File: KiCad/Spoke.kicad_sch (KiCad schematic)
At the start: 134 parts, among them J1 B2B-PH-K-S, J10 BL-A, J11 BL-C, J12 Amphenol 132289, J2 BAT+, J3 BAT-, J4 GCT USB4105/USB4110, J5 USB+, J6 USB-, J7 PLS-1x3, J8 PLS-1x6, J9 PLS-1x3, Q1 AO3407A, Q2 AO3407A, Q3 AO3400, Q4 AO3400, Q5 AO3400, SW1 PWR, SW2 OK/UP, SW3 ESC/DN, SW4 BOOT, U1 SP0503BAHTG, U2 TP4056, U3 CP2102N-A02-GQFN28, U4 LM3671MF-3.3, U5 74HC4052PW, U6 STM32F103C8T6, U7 LSM303DLHC, X1 8MHz

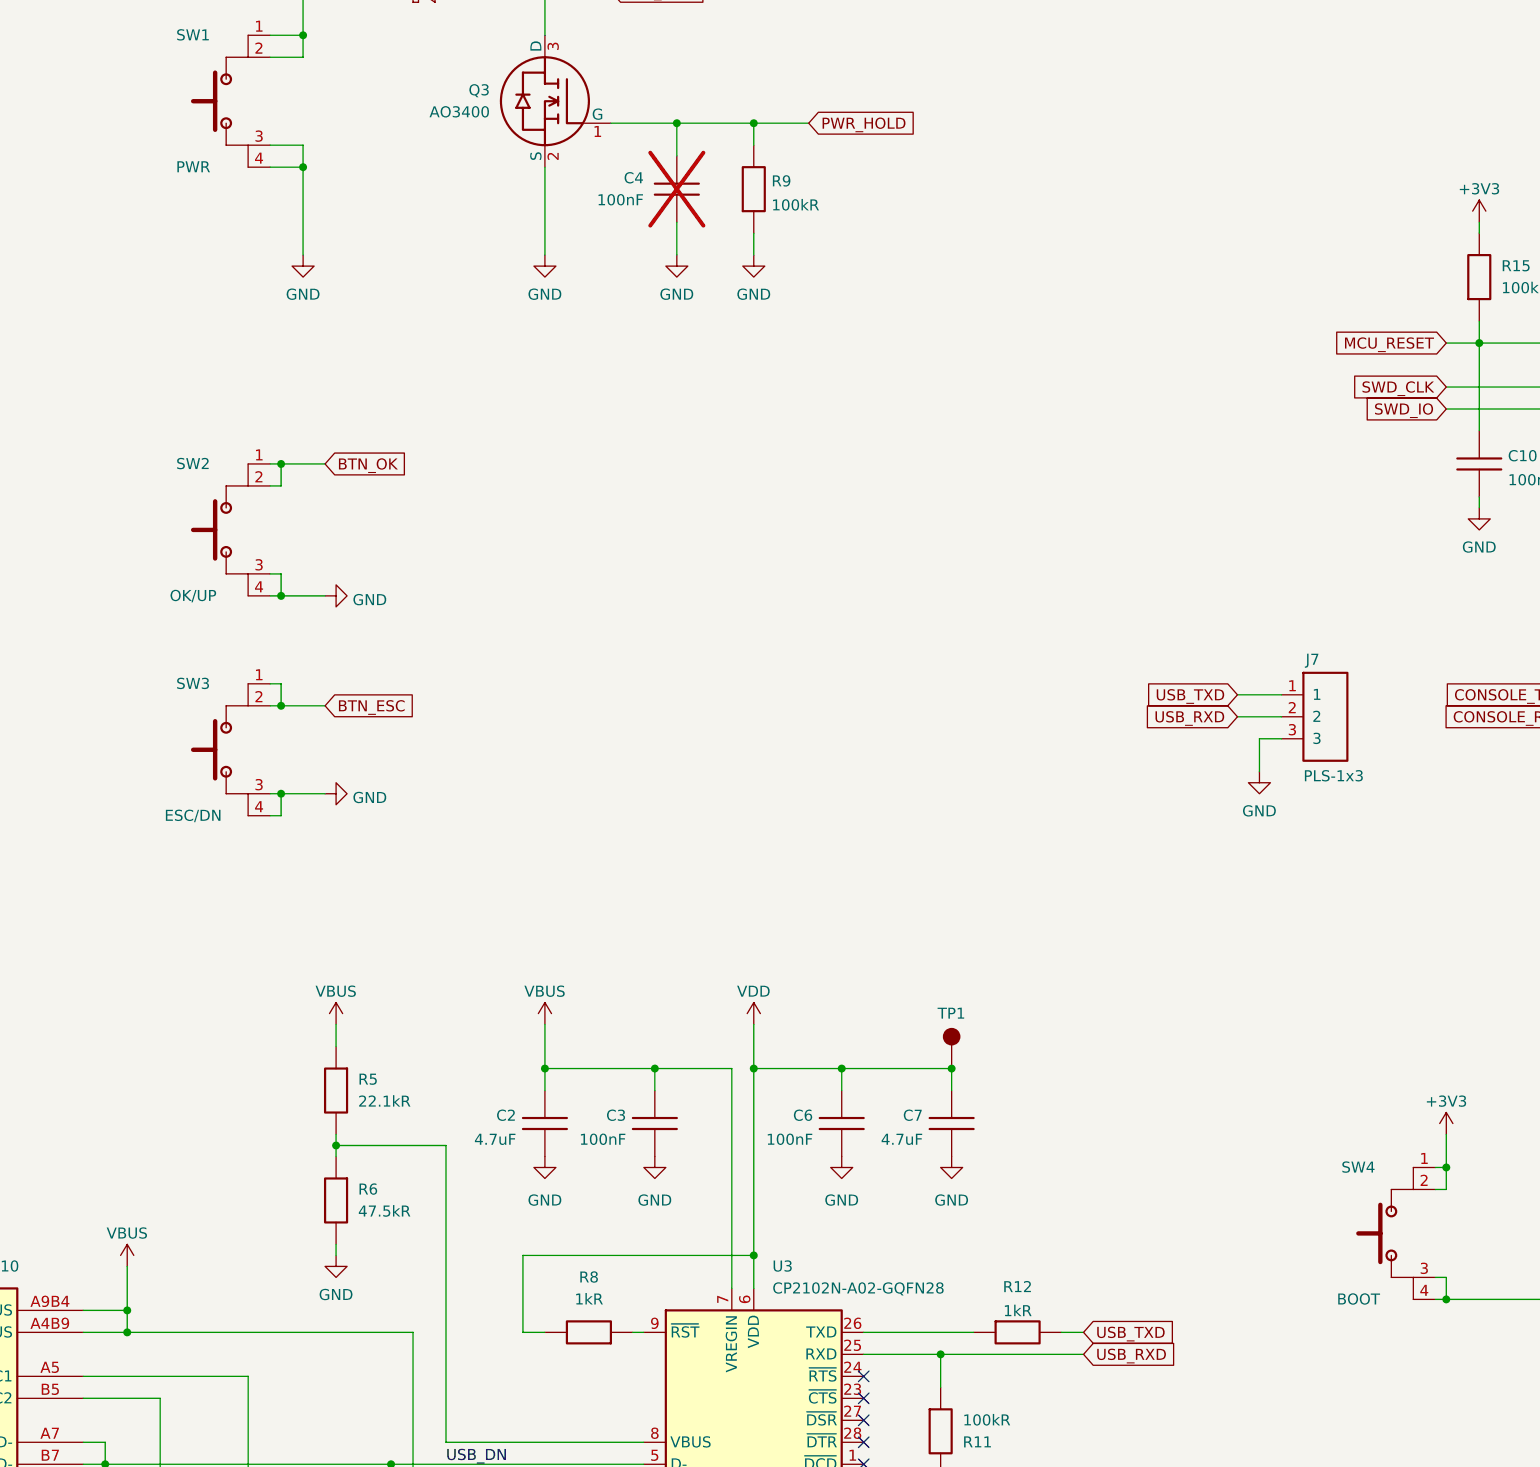
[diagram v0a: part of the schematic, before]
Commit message: Export SCH and BOM
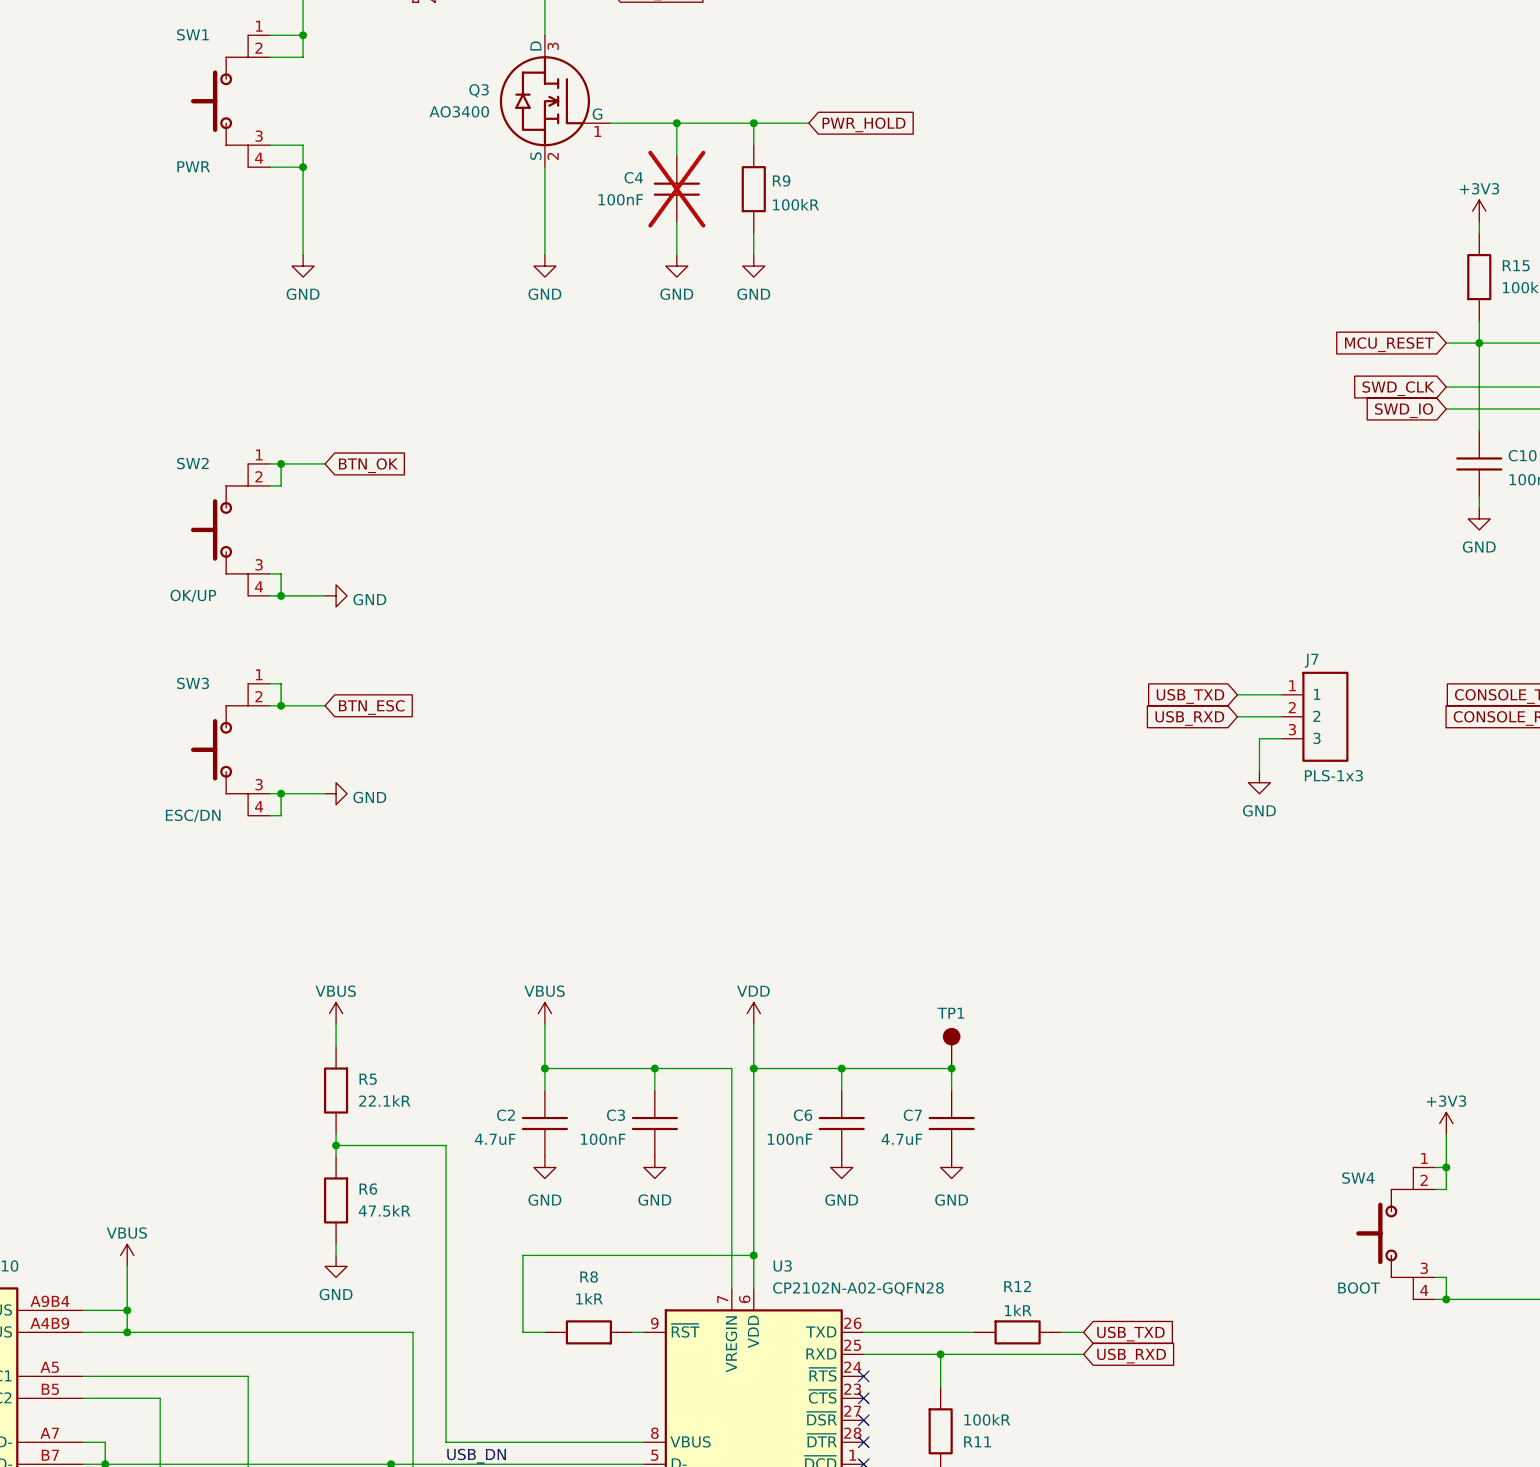
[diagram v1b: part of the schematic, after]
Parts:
- J10, J11, J2, J3, J5, J6, TP1, TP10, TP11, TP12, TP13, TP14, TP15, TP16, TP17, TP18, TP2, TP3, TP4, TP5, TP6, TP7, TP8, TP9: now left out of the parts list
- SW1: value PWR -> ~
- SW2: value OK/UP -> ~
- SW3: value ESC/DN -> ~
- SW4: value BOOT -> ~
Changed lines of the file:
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@@
 		(unit 1)
 		(exclude_from_sim no)
-		(in_bom yes)
+		(in_bom no)
 		(on_board yes)
 		(dnp no)
@@
 		)
 		(property "Description" ""
-			(at 346.71 203.2 0)
+			(at 341.63 207.01 0)
 			(effects
 				(font
@@
 		(unit 1)
 		(exclude_from_sim no)
-		(in_bom yes)
+		(in_bom no)
 		(on_board yes)
 		(dnp no)
@@
 		(unit 1)
 		(exclude_from_sim no)
-		(in_bom yes)
+		(in_bom no)
 		(on_board yes)
 		(dnp no)
@@
 		(unit 1)
 		(exclude_from_sim no)
-		(in_bom yes)
+		(in_bom no)
 		(on_board yes)
 		(dnp no)
@@
 		(unit 1)
 		(exclude_from_sim no)
-		(in_bom yes)
+		(in_bom no)
 		(on_board yes)
 		(dnp no)
@@
 		(unit 1)
 		(exclude_from_sim no)
-		(in_bom yes)
+		(in_bom no)
 		(on_board yes)
 		(dnp no)
@@
 		)
 		(property "Value" "~"
-			(at 236.22 58.42 0)
+			(at 236.22 67.31 0)
 			(effects
 				(font
@@
 		(unit 1)
 		(exclude_from_sim no)
-		(in_bom yes)
+		(in_bom no)
 		(on_board yes)
 		(dnp no)
@@
 		(unit 1)
 		(exclude_from_sim no)
-		(in_bom yes)
+		(in_bom no)
 		(on_board yes)
 		(dnp no)
@@
 		)
 		(property "Description" ""
-			(at 134.62 349.25 0)
+			(at 139.7 353.06 0)
 			(effects
 				(font
@@
 		(unit 1)
 		(exclude_from_sim no)
-		(in_bom yes)
+		(in_bom no)
 		(on_board yes)
 		(dnp no)
@@
 		(unit 1)
 		(exclude_from_sim no)
-		(in_bom yes)
+		(in_bom no)
 		(on_board yes)
 		(dnp no)
@@
 		(unit 1)
 		(exclude_from_sim no)
-		(in_bom yes)
+		(in_bom no)
 		(on_board yes)
 		(dnp no)
@@
 		(unit 1)
 		(exclude_from_sim no)
-		(in_bom yes)
+		(in_bom no)
 		(on_board yes)
 		(dnp no)
@@
 		(unit 1)
 		(exclude_from_sim no)
-		(in_bom yes)
+		(in_bom no)
 		(on_board yes)
 		(dnp no)
@@
 			)
 		)
-		(property "Value" "OK/UP"
+		(property "Value" "~"
 			(at 72.39 143.51 0)
 			(effects
@@
 					(size 1.27 1.27)
 				)
+				(hide yes)
 			)
 		)
@@
 			)
 		)
-		(property "Description" ""
-			(at 81.28 130.81 0)
+		(property "Description" "OK/UP"
+			(at 72.39 143.51 0)
 			(effects
 				(font
 					(size 1.27 1.27)
 				)
-				(hide yes)
 			)
 		)
@@
 		(unit 1)
 		(exclude_from_sim no)
-		(in_bom yes)
+		(in_bom no)
 		(on_board yes)
 		(dnp no)
@@
 			)
 		)
-		(property "Value" "ESC/DN"
+		(property "Value" "~"
 			(at 72.39 168.91 0)
 			(effects
@@
 					(size 1.27 1.27)
 				)
+				(hide yes)
 			)
 		)
@@
 			)
 		)
-		(property "Description" ""
-			(at 81.28 156.21 0)
+		(property "Description" "ESC/DN"
+			(at 72.39 168.91 0)
 			(effects
 				(font
 					(size 1.27 1.27)
 				)
-				(hide yes)
 			)
 		)
@@
 		(unit 1)
 		(exclude_from_sim no)
-		(in_bom yes)
+		(in_bom no)
 		(on_board yes)
 		(dnp no)
@@
 		(unit 1)
 		(exclude_from_sim no)
-		(in_bom yes)
+		(in_bom no)
 		(on_board yes)
 		(dnp no)
@@
 		(dnp no)
 		(property "Reference" "SW4"
-			(at 207.01 209.55 0)
+			(at 207.01 210.82 0)
 			(effects
 				(font
@@
 			)
 		)
-		(property "Value" "BOOT"
+		(property "Value" "~"
 			(at 207.01 224.79 0)
 			(effects
@@
 					(size 1.27 1.27)
 				)
+				(hide yes)
 			)
 		)
@@
 			)
 		)
-		(property "Description" ""
-			(at 215.9 212.09 0)
+		(property "Description" "BOOT"
+			(at 207.01 223.52 0)
 			(effects
 				(font
 					(size 1.27 1.27)
 				)
-				(hide yes)
 			)
 		)
@@
 		)
 		(property "Description" ""
-			(at 346.71 215.9 0)
+			(at 341.63 219.71 0)
 			(effects
 				(font
@@
 		(unit 1)
 		(exclude_from_sim no)
-		(in_bom yes)
+		(in_bom no)
 		(on_board yes)
 		(dnp no)
@@
 		(unit 1)
 		(exclude_from_sim no)
-		(in_bom yes)
+		(in_bom no)
 		(on_board yes)
 		(dnp no)
@@
 		(unit 1)
 		(exclude_from_sim no)
-		(in_bom yes)
+		(in_bom no)
 		(on_board yes)
 		(dnp no)
@@
 		(unit 1)
 		(exclude_from_sim no)
-		(in_bom yes)
+		(in_bom no)
 		(on_board yes)
 		(dnp no)
@@
 			)
 		)
-		(property "Value" "PWR"
+		(property "Value" "~"
 			(at 72.39 93.98 0)
 			(effects
@@
 					(size 1.27 1.27)
 				)
+				(hide yes)
 			)
 		)
@@
 			)
 		)
-		(property "Description" ""
-			(at 81.28 81.28 0)
+		(property "Description" "PWR"
+			(at 72.39 93.98 0)
 			(effects
 				(font
 					(size 1.27 1.27)
 				)
-				(hide yes)
 			)
 		)
@@
 		(unit 1)
 		(exclude_from_sim no)
-		(in_bom yes)
+		(in_bom no)
 		(on_board yes)
 		(dnp no)
@@
 		(unit 1)
 		(exclude_from_sim no)
-		(in_bom yes)
+		(in_bom no)
 		(on_board yes)
 		(dnp no)
@@
 		(unit 1)
 		(exclude_from_sim no)
-		(in_bom yes)
+		(in_bom no)
 		(on_board yes)
 		(dnp no)
@@
 		(unit 1)
 		(exclude_from_sim no)
-		(in_bom yes)
+		(in_bom no)
 		(on_board yes)
 		(dnp no)
